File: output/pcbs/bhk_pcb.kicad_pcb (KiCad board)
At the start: 2 copper layers, 164.2 x 123.2 mm, 116 parts

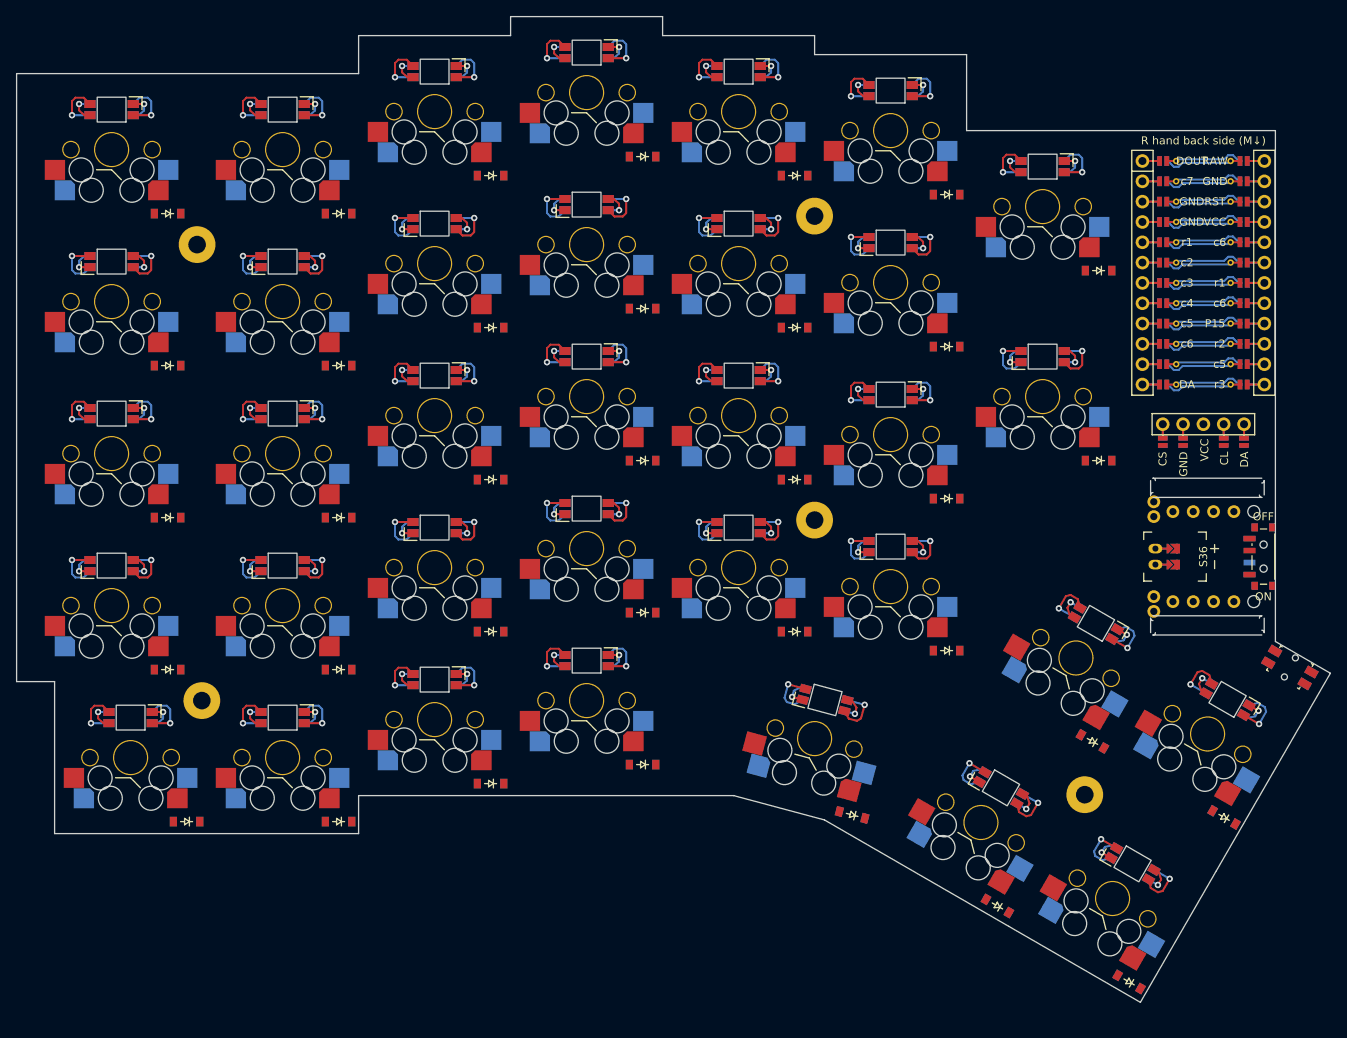
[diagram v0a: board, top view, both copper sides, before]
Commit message: fix ed some routing
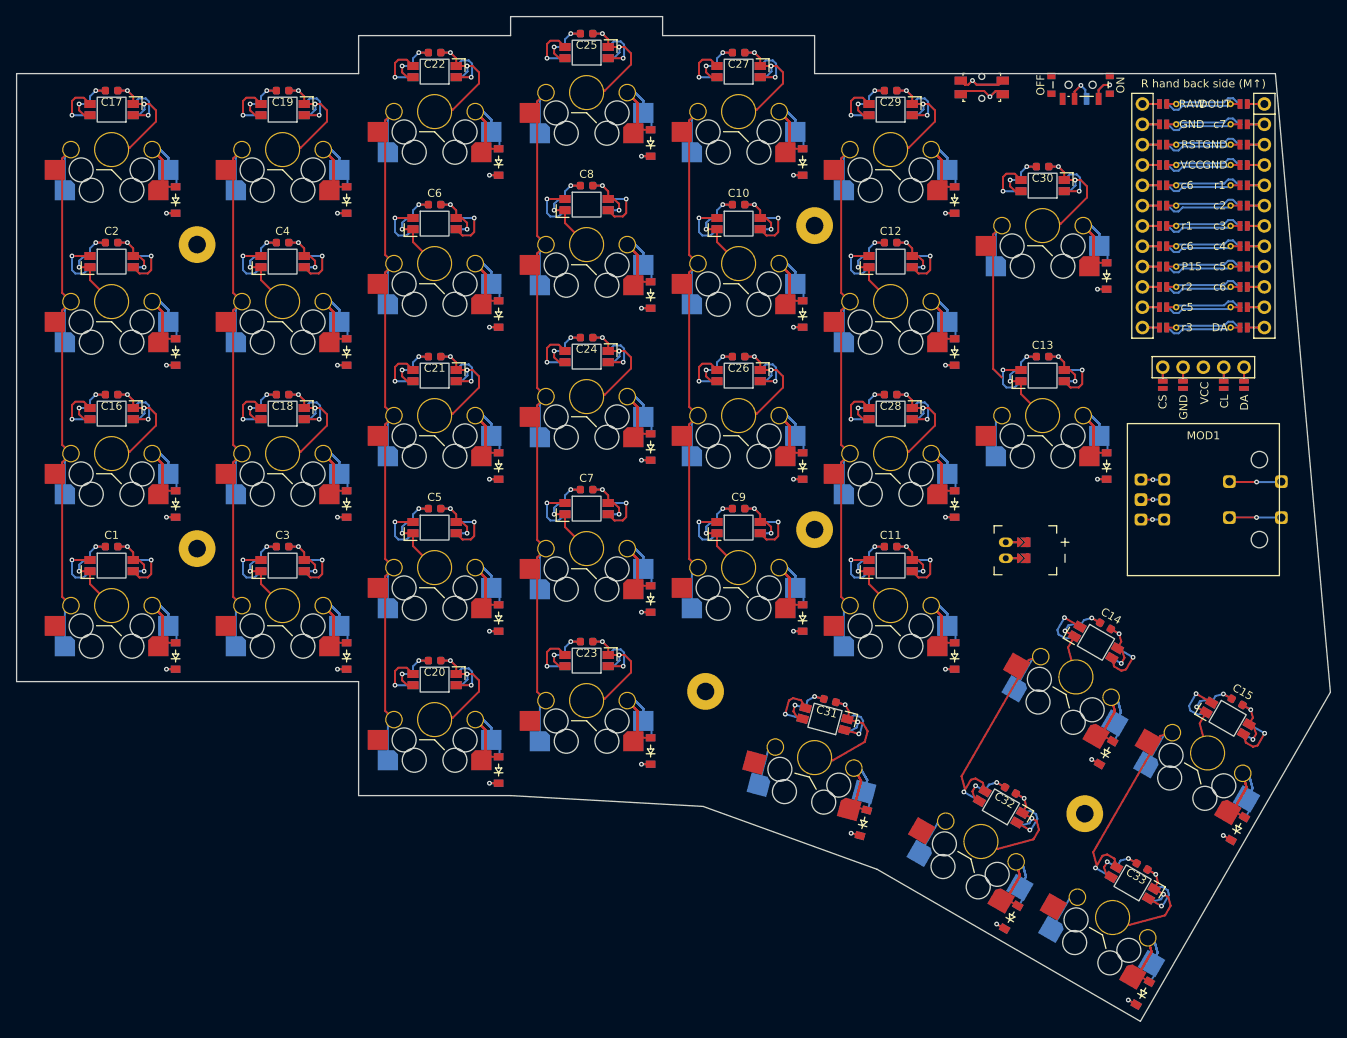
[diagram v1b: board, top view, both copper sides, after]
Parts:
- removed D34, D35: , ceoloide:diode_tht_sod123
- removed LED34, LED35: , ceoloide:led_SK6812mini-e (per-key, reversible)
- removed S34, S35: , ceoloide:switch_mx
- removed S36: RollerEncoder_Panasonic_EVQWGD001, bhkfp:scrollwheel
- added C1: Capacitor_0603, Capacitor_0603, F.Cu at (150.0, 123.6)
- added C10: Capacitor_0603, Capacitor_0603, F.Cu at (228.4, 80.9)
- added C11: Capacitor_0603, Capacitor_0603, F.Cu at (247.4, 123.6)
- added C12: Capacitor_0603, Capacitor_0603, F.Cu at (247.4, 85.6)
- added C13: Capacitor_0603, Capacitor_0603, F.Cu at (266.4, 99.9)
- added C14: Capacitor_0603, Capacitor_0603, F.Cu at (274.2, 133.5)
- added C15: Capacitor_0603, Capacitor_0603, F.Cu at (290.7, 143.0)
- added C16: Capacitor_0603, Capacitor_0603, F.Cu at (150.0, 104.6)
- added C17: Capacitor_0603, Capacitor_0603, F.Cu at (150.0, 66.6)
- added C18: Capacitor_0603, Capacitor_0603, F.Cu at (171.4, 104.6)
- added C19: Capacitor_0603, Capacitor_0603, F.Cu at (171.4, 66.6)
- added C2: Capacitor_0603, Capacitor_0603, F.Cu at (150.0, 85.6)
- added C20: Capacitor_0603, Capacitor_0603, F.Cu at (190.4, 137.9)
- added C21: Capacitor_0603, Capacitor_0603, F.Cu at (190.4, 99.9)
- added C22: Capacitor_0603, Capacitor_0603, F.Cu at (190.4, 61.9)
- added C23: Capacitor_0603, Capacitor_0603, F.Cu at (209.4, 135.5)
- added C24: Capacitor_0603, Capacitor_0603, F.Cu at (209.4, 97.5)
- added C25: Capacitor_0603, Capacitor_0603, F.Cu at (209.4, 59.5)
- added C26: Capacitor_0603, Capacitor_0603, F.Cu at (228.4, 99.9)
- added C27: Capacitor_0603, Capacitor_0603, F.Cu at (228.4, 61.9)
- added C28: Capacitor_0603, Capacitor_0603, F.Cu at (247.4, 104.6)
- added C29: Capacitor_0603, Capacitor_0603, F.Cu at (247.4, 66.6)
- added C3: Capacitor_0603, Capacitor_0603, F.Cu at (171.4, 123.6)
- added C30: Capacitor_0603, Capacitor_0603, F.Cu at (266.4, 76.1)
- added C31: Capacitor_0603, Capacitor_0603, F.Cu at (239.8, 142.9)
- added C32: Capacitor_0603, Capacitor_0603, F.Cu at (262.4, 154.1)
- added C33: Capacitor_0603, Capacitor_0603, F.Cu at (278.8, 163.6)
- added C4: Capacitor_0603, Capacitor_0603, F.Cu at (171.4, 85.6)
- added C5: Capacitor_0603, Capacitor_0603, F.Cu at (190.4, 118.9)
- added C6: Capacitor_0603, Capacitor_0603, F.Cu at (190.4, 80.9)
- added C7: Capacitor_0603, Capacitor_0603, F.Cu at (209.4, 116.5)
- added C8: Capacitor_0603, Capacitor_0603, F.Cu at (209.4, 78.5)
- added C9: Capacitor_0603, Capacitor_0603, F.Cu at (228.4, 118.9)
- added H6: , ceoloide:mounting_hole_plated, F.Cu at (224.2, 141.7)
- added MOD1: , THQWGD001C, F.Cu at (286.5, 117.8)
- JST1: moved to B.Cu
- moved LED16 139.5 mm to (150.0, 107.0), turned to 180 degrees
- moved LED32 90.6 mm to (261.2, 156.2), turned to 150 degrees
- moved LED33 90.2 mm to (277.6, 165.7), turned to 150 degrees
- moved RST1 82.1 mm to (258.8, 66.2), turned to 0 degrees
- moved D30 81.6 mm to (262.4, 169.9), turned to 60 degrees
- moved S30 79.7 mm to (258.7, 160.5), turned to 150 degrees
- moved LED17 76.0 mm to (150.0, 69.0)
- moved PWR1 63.2 mm to (271.1, 65.9), turned to 90 degrees
- moved S5 60.9 mm to (171.4, 131.0)
- moved D5 59.7 mm to (179.4, 137.3), turned to 90 degrees
- moved LED28 59.0 mm to (247.4, 107.0)
- moved S14 57.8 mm to (209.4, 142.9)
- moved S15 57.8 mm to (209.4, 123.9)
- moved D14 56.6 mm to (217.4, 149.2), turned to 90 degrees
- moved D15 56.6 mm to (217.4, 130.2), turned to 90 degrees
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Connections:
- D1 pad 1: r5 -> r4
- D1 pad 2: c1_r5 -> c1_r4
- D10 pad 1: r1 -> r4
- D10 pad 2: c2_r1 -> c3_r4
- D11 pad 1: r5 -> r3
- D11 pad 2: c3_r5 -> c3_r3
- D12 pad 1: r4 -> r2
- D12 pad 2: c3_r4 -> c3_r2
- D13 pad 1: r3 -> r1
- D13 pad 2: c3_r3 -> c3_r1
- D14 pad 1: r2 -> r5
- D14 pad 2: c3_r2 -> c4_r5
- D15 pad 1: r1 -> r4
- D15 pad 2: c3_r1 -> c4_r4
- D16 pad 1: r5 -> r3
- D16 pad 2: c4_r5 -> c4_r3
- D17 pad 1: r4 -> r2
- D17 pad 2: c4_r4 -> c4_r2
- D18 pad 1: r3 -> r1
- D18 pad 2: c4_r3 -> c4_r1
- D19 pad 1: r2 -> r4
- D19 pad 2: c4_r2 -> c5_r4
- D2 pad 1: r4 -> r3
- D2 pad 2: c1_r4 -> c1_r3
- D20 pad 1: r1 -> r3
- D20 pad 2: c4_r1 -> c5_r3
- D21 pad 1: r4 -> r2
- D21 pad 2: c5_r4 -> c5_r2
- D22 pad 1: r3 -> r1
- D22 pad 2: c5_r3 -> c5_r1
- D23 pad 1: r2 -> r4
- D23 pad 2: c5_r2 -> c6_r4
- D24 pad 1: r1 -> r3
- D24 pad 2: c5_r1 -> c6_r3
- D25 pad 1: r4 -> r2
- D25 pad 2: c6_r4 -> c6_r2
- D26 pad 1: r3 -> r1
- D26 pad 2: c6_r3 -> c6_r1
- D27 pad 2: c6_r2 -> c7_r2
- D28 pad 2: c6_r1 -> c7_r1
- D29 pad 1: r2 -> r5
- D29 pad 2: c7_r2 -> c1_r2
- D3 pad 1: r3 -> r2
- D3 pad 2: c1_r3 -> c1_r2
- D30 pad 1: r1 -> r5
- D30 pad 2: c7_r1 -> c2_r2
- D31 pad 1: r5 -> r3
- D31 pad 2: c1_r2 -> c2_r1
- D32 pad 2: c2_r2 -> c3_r2
- D33 pad 1: r3 -> r4
- D33 pad 2: c2_r1 -> c3_r1
- D4 pad 1: r2 -> r1
- D4 pad 2: c1_r2 -> c1_r1
- D5 pad 1: r1 -> r4
- D5 pad 2: c1_r1 -> c2_r4
- D6 pad 1: r5 -> r3
- D6 pad 2: c2_r5 -> c2_r3
- D7 pad 1: r4 -> r2
- D7 pad 2: c2_r4 -> c2_r2
- D8 pad 1: r3 -> r1
- D8 pad 2: c2_r3 -> c2_r1
- D9 pad 1: r2 -> r5
- D9 pad 2: c2_r2 -> c3_r5
- LED14 pad 2: LED_31 -> LED_27
- LED14 pad 4: LED_30 -> LED_26
- LED15 pad 2: LED_32 -> LED_28
- LED15 pad 4: LED_31 -> LED_27
- LED16 pad 2: LED_34 -> LED_20
- LED16 pad 4: LED_33 -> LED_19
- LED17 pad 2: LED_27 -> LED_7
- LED17 pad 4: LED_26 -> LED_6
- LED18 pad 2: LED_15 -> LED_19
- LED18 pad 4: LED_14 -> LED_18
- LED19 pad 2: LED_7 -> LED_6
- LED19 pad 4: LED_6 -> LED_5
- LED20 pad 2: LED_28 -> LED_END
- LED20 pad 4: LED_27 -> LED_32
- LED21 pad 2: LED_16 -> LED_18
- LED21 pad 4: LED_15 -> LED_17
- LED22 pad 2: LED_6 -> LED_5
- LED22 pad 4: LED_5 -> LED_4
- LED23 pad 2: LED_29 -> LED_32
- LED23 pad 4: LED_28 -> LED_31
- LED25 pad 2: LED_5 -> LED_4
- LED25 pad 4: LED_4 -> LED_3
- LED26 pad 2: LED_30 -> LED_16
- LED26 pad 4: LED_29 -> LED_15
- LED27 pad 2: LED_18 -> LED_3
- LED27 pad 4: LED_17 -> LED_2
- LED28 pad 2: LED_4 -> LED_15
- LED28 pad 4: LED_3 -> LED_14
- LED29 pad 2: LED_19 -> LED_2
- LED29 pad 4: LED_18 -> LED_1
- LED30 pad 2: LED_3 -> LED_1
- LED30 pad 4: LED_2 -> DOUT
- LED31 pad 2: LED_20 -> LED_31
- LED31 pad 4: LED_19 -> LED_30
- LED32 pad 2: LED_2 -> LED_30
- LED32 pad 4: LED_1 -> LED_29
- LED33 pad 2: LED_1 -> LED_29
- LED33 pad 4: DOUT -> LED_28
- MCU1 pad 101: RAW -> DOUT
- MCU1 pad 102: GND -> c7
- MCU1 pad 103: RST -> GND
- MCU1 pad 104: VCC -> GND
- MCU1 pad 105: c6 -> r1
- MCU1 pad 106: (no net) -> c2
- MCU1 pad 107: r1 -> c3
- MCU1 pad 108: c6 -> c4
- MCU1 pad 109: P15 -> c5
- MCU1 pad 110: r2 -> c6
- MCU1 pad 111: c5 -> (no net)
- MCU1 pad 112: r3 -> DA
- MCU1 pad 113: DA -> r3
- MCU1 pad 114: (no net) -> c5
- MCU1 pad 115: c6 -> r2
- MCU1 pad 116: c5 -> P15
- MCU1 pad 117: c4 -> c6
- MCU1 pad 118: c3 -> r1
- MCU1 pad 119: c2 -> (no net)
- MCU1 pad 120: r1 -> c6
- MCU1 pad 121: GND -> VCC
- MCU1 pad 122: GND -> RST
- MCU1 pad 123: c7 -> GND
- MCU1 pad 124: DOUT -> RAW
- S1 pad : c1_r5 -> c1_r4
- S1 pad 1: c1_r5 -> c1_r4
- S10 pad : c2_r1 -> c3_r4
- S10 pad 1: c2_r1 -> c3_r4
- S10 pad 2: c2 -> c3
- S11 pad : c3_r5 -> c3_r3
- S11 pad 1: c3_r5 -> c3_r3
- S12 pad : c3_r4 -> c3_r2
- S12 pad 1: c3_r4 -> c3_r2
- S13 pad : c3_r3 -> c3_r1
- S13 pad 1: c3_r3 -> c3_r1
- S14 pad : c3_r2 -> c4_r5
- S14 pad 1: c3_r2 -> c4_r5
- S14 pad 2: c3 -> c4
- S15 pad : c3_r1 -> c4_r4
- S15 pad 1: c3_r1 -> c4_r4
- S15 pad 2: c3 -> c4
- S16 pad : c4_r5 -> c4_r3
- S16 pad 1: c4_r5 -> c4_r3
- S17 pad : c4_r4 -> c4_r2
- S17 pad 1: c4_r4 -> c4_r2
- S18 pad : c4_r3 -> c4_r1
- S18 pad 1: c4_r3 -> c4_r1
- S19 pad : c4_r2 -> c5_r4
- S19 pad 1: c4_r2 -> c5_r4
- S19 pad 2: c4 -> c5
- S2 pad : c1_r4 -> c1_r3
- S2 pad 1: c1_r4 -> c1_r3
- S20 pad : c4_r1 -> c5_r3
- S20 pad 1: c4_r1 -> c5_r3
- S20 pad 2: c4 -> c5
- S21 pad : c5_r4 -> c5_r2
- S21 pad 1: c5_r4 -> c5_r2
- S22 pad : c5_r3 -> c5_r1
- S22 pad 1: c5_r3 -> c5_r1
- S23 pad : c5_r2 -> c6_r4
- S23 pad 1: c5_r2 -> c6_r4
- S23 pad 2: c5 -> c6
- S24 pad : c5_r1 -> c6_r3
- S24 pad 1: c5_r1 -> c6_r3
- S24 pad 2: c5 -> c6
- S25 pad : c6_r4 -> c6_r2
- S25 pad 1: c6_r4 -> c6_r2
- S26 pad : c6_r3 -> c6_r1
- S26 pad 1: c6_r3 -> c6_r1
- S27 pad : c6_r2 -> c7_r2
- S27 pad 1: c6_r2 -> c7_r2
- S27 pad 2: c6 -> c7
- S28 pad : c6_r1 -> c7_r1
- S28 pad 1: c6_r1 -> c7_r1
- S28 pad 2: c6 -> c7
- S29 pad : c7_r2 -> c1_r2
- S29 pad 1: c7_r2 -> c1_r2
- S29 pad 2: c7 -> c5
- S3 pad : c1_r3 -> c1_r2
- S3 pad 1: c1_r3 -> c1_r2
- S30 pad : c7_r1 -> c2_r2
- S30 pad 1: c7_r1 -> c2_r2
- S30 pad 2: c7 -> c6
- S31 pad : c1_r2 -> c2_r1
- S31 pad 1: c1_r2 -> c2_r1
- S31 pad 2: c5 -> c7
- S32 pad : c2_r2 -> c3_r2
- S32 pad 1: c2_r2 -> c3_r2
- S32 pad 2: c6 -> c7
- S33 pad : c2_r1 -> c3_r1
- S33 pad 1: c2_r1 -> c3_r1
- S4 pad : c1_r2 -> c1_r1
- S4 pad 1: c1_r2 -> c1_r1
- S5 pad : c1_r1 -> c2_r4
- S5 pad 1: c1_r1 -> c2_r4
- S5 pad 2: c1 -> c2
- S6 pad : c2_r5 -> c2_r3
- S6 pad 1: c2_r5 -> c2_r3
- S7 pad : c2_r4 -> c2_r2
- S7 pad 1: c2_r4 -> c2_r2
- S8 pad : c2_r3 -> c2_r1
- S8 pad 1: c2_r3 -> c2_r1
- S9 pad : c2_r2 -> c3_r5
- S9 pad 1: c2_r2 -> c3_r5
- S9 pad 2: c2 -> c3
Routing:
- net (no net): track 333.1 -> 3412.2 mm, vias 0 -> 240
- net VCC: track 131.4 -> 0.00 mm, vias 35 -> 0
- net GND: track 131.4 -> 0.00 mm, vias 35 -> 0
- net LED_29: track 13.5 -> 0.00 mm, vias 2 -> 0
- net LED_28: track 13.5 -> 0.00 mm, vias 2 -> 0
- net LED_27: track 13.5 -> 0.00 mm, vias 2 -> 0
- net LED_26: track 13.5 -> 0.00 mm, vias 2 -> 0
- net LED_9: track 13.5 -> 0.00 mm, vias 2 -> 0
- net LED_8: track 13.5 -> 0.00 mm, vias 2 -> 0
- net LED_7: track 13.5 -> 0.00 mm, vias 2 -> 0
- net LED_6: track 13.5 -> 0.00 mm, vias 2 -> 0
- net LED_5: track 13.5 -> 0.00 mm, vias 2 -> 0
- net LED_4: track 13.5 -> 0.00 mm, vias 2 -> 0
- net LED_3: track 13.5 -> 0.00 mm, vias 2 -> 0
- net LED_25: track 13.5 -> 0.00 mm, vias 2 -> 0
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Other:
- board size 164.2 x 123.2 mm -> 164.2 x 125.6 mm
